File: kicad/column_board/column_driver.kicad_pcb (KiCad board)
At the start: 2 copper layers, 100 x 100 mm, 104 parts, among them J1 Panel column connector (femal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, J2 PWR_CHAIN_IN, J3 PWR_CHAIN_OUT, J4 DATA_CHAIN_IN, J5 DATA_CHAIN_OUT, U1 TPIC6B595, U10 TPIC6B595, U11 TPIC6B595, U12 TBD62783, U2 TPIC6B595, U3 TBD62783, U4 TPIC6B595, U5 TPIC6B595, U6 TBD62783, U7 TPIC6B595, U8 TPIC6B595, U9 TBD62783

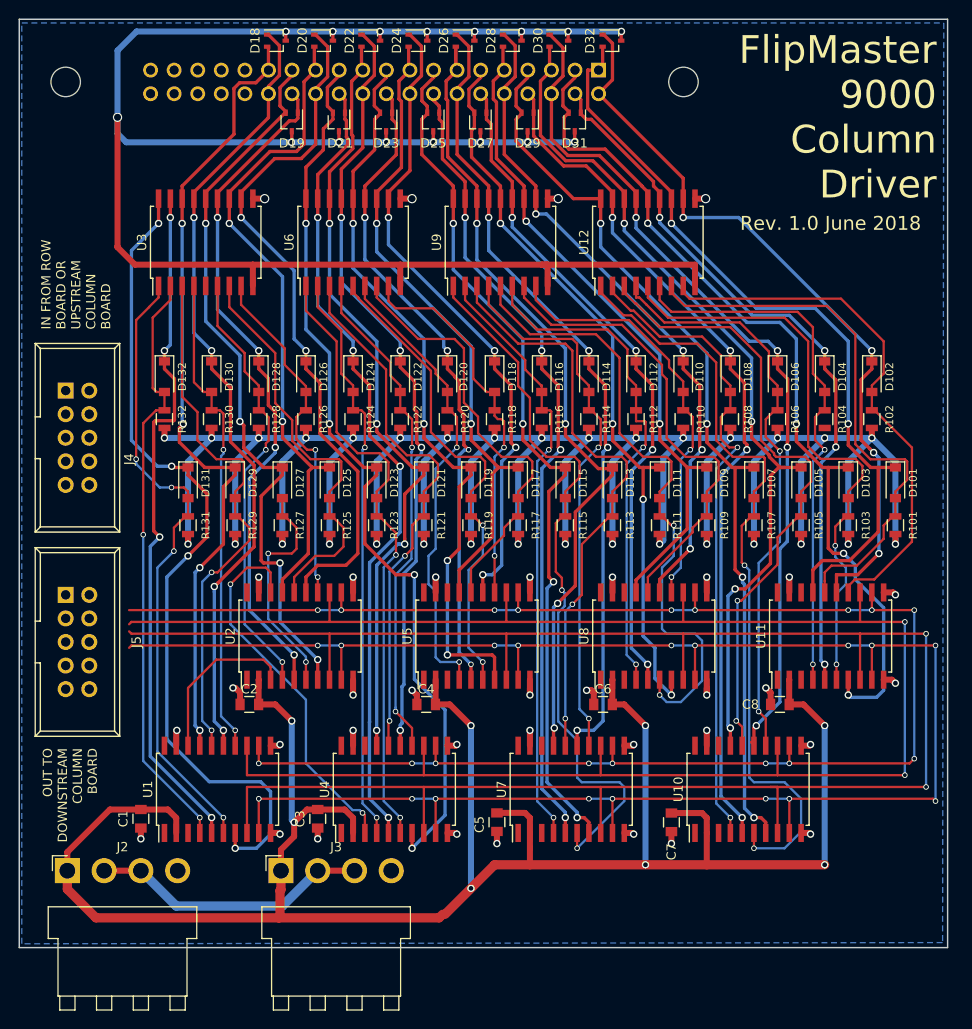
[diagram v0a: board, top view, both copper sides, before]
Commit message: Nearly done routing column board.
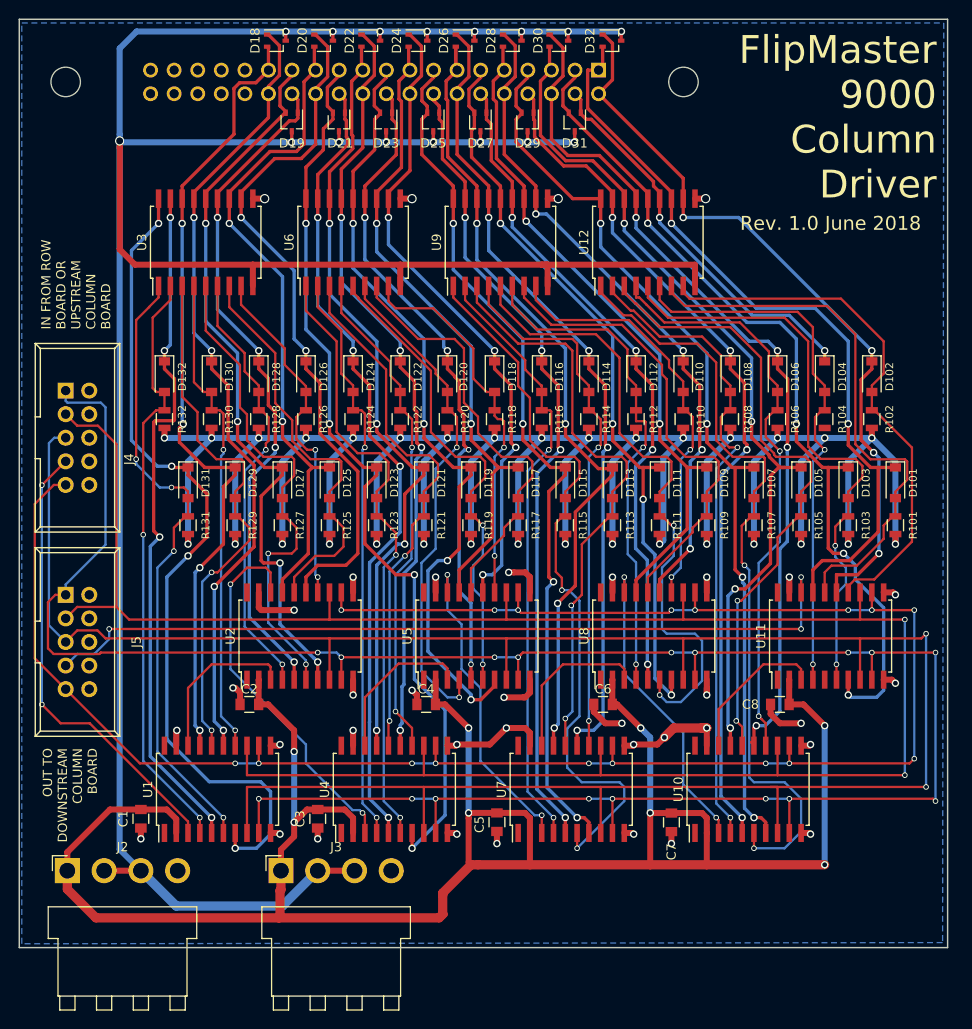
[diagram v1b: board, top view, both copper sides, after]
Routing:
- net RC_DATA_OUT: track 0.00 -> 88.7 mm, vias 0 -> 3
- net +24V: track 246.9 -> 324.0 mm
- net RC_DATA: track 0.00 -> 49.4 mm, vias 0 -> 2
- net ~COL_EN: track 206.2 -> 245.6 mm
- net COL4: track 79.1 -> 43.3 mm, vias 4 -> 2
- net Net-(U5-Pad18): track 0.00 -> 34.4 mm, vias 0 -> 2
- net Net-(U10-Pad3): track 0.00 -> 33.4 mm, vias 0 -> 2
- net GND: track 54.0 -> 85.6 mm, vias 36 -> 37
- net RC_SHIFT_CLK: track 196.5 -> 227.8 mm
- net ~RC_CLEAR: track 216.0 -> 246.0 mm
- net Net-(D127-Pad2): track 25.5 -> 54.6 mm
- net COL_REG_CLK: track 186.7 -> 213.7 mm
- net Net-(U7-Pad18): track 0.00 -> 17.7 mm
- net Net-(U4-Pad18): track 0.00 -> 17.0 mm
- net Net-(U10-Pad18): track 0.00 -> 16.2 mm
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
